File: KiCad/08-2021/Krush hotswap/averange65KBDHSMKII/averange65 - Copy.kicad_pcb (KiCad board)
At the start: 2 copper layers, 303.2 x 98.7 mm, 200 parts, among them SW1 SW_Push, SW2 Rotary_Encoder_Switch, U1 PRTR5V0U2X, U2 ATmega32U4-MU, U4 STF202-22T1G, Y1 Crystal_GND2

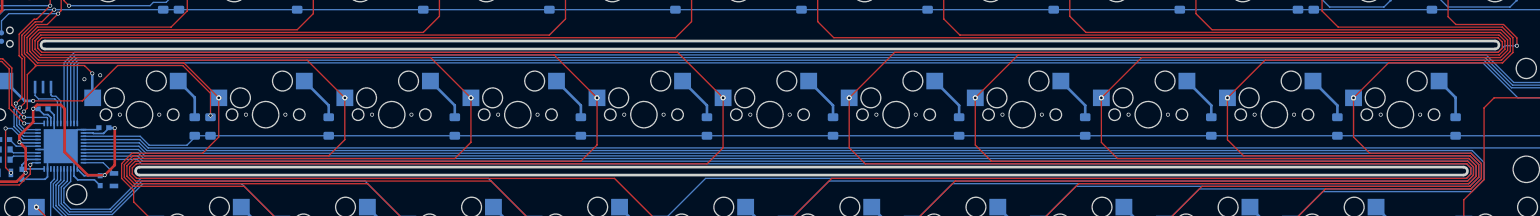
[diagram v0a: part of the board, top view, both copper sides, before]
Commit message: a
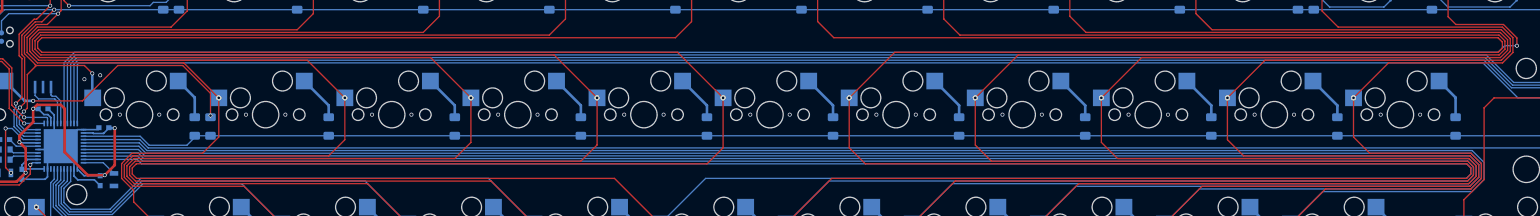
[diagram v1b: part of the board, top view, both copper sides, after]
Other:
- outline, holes or cut-outs redrawn
